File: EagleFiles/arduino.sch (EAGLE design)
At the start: 41 parts, among them IC1 4067D, IC2 4067D, IC3 4067D, J1 AVR_SPI, U1 ATMEGA168

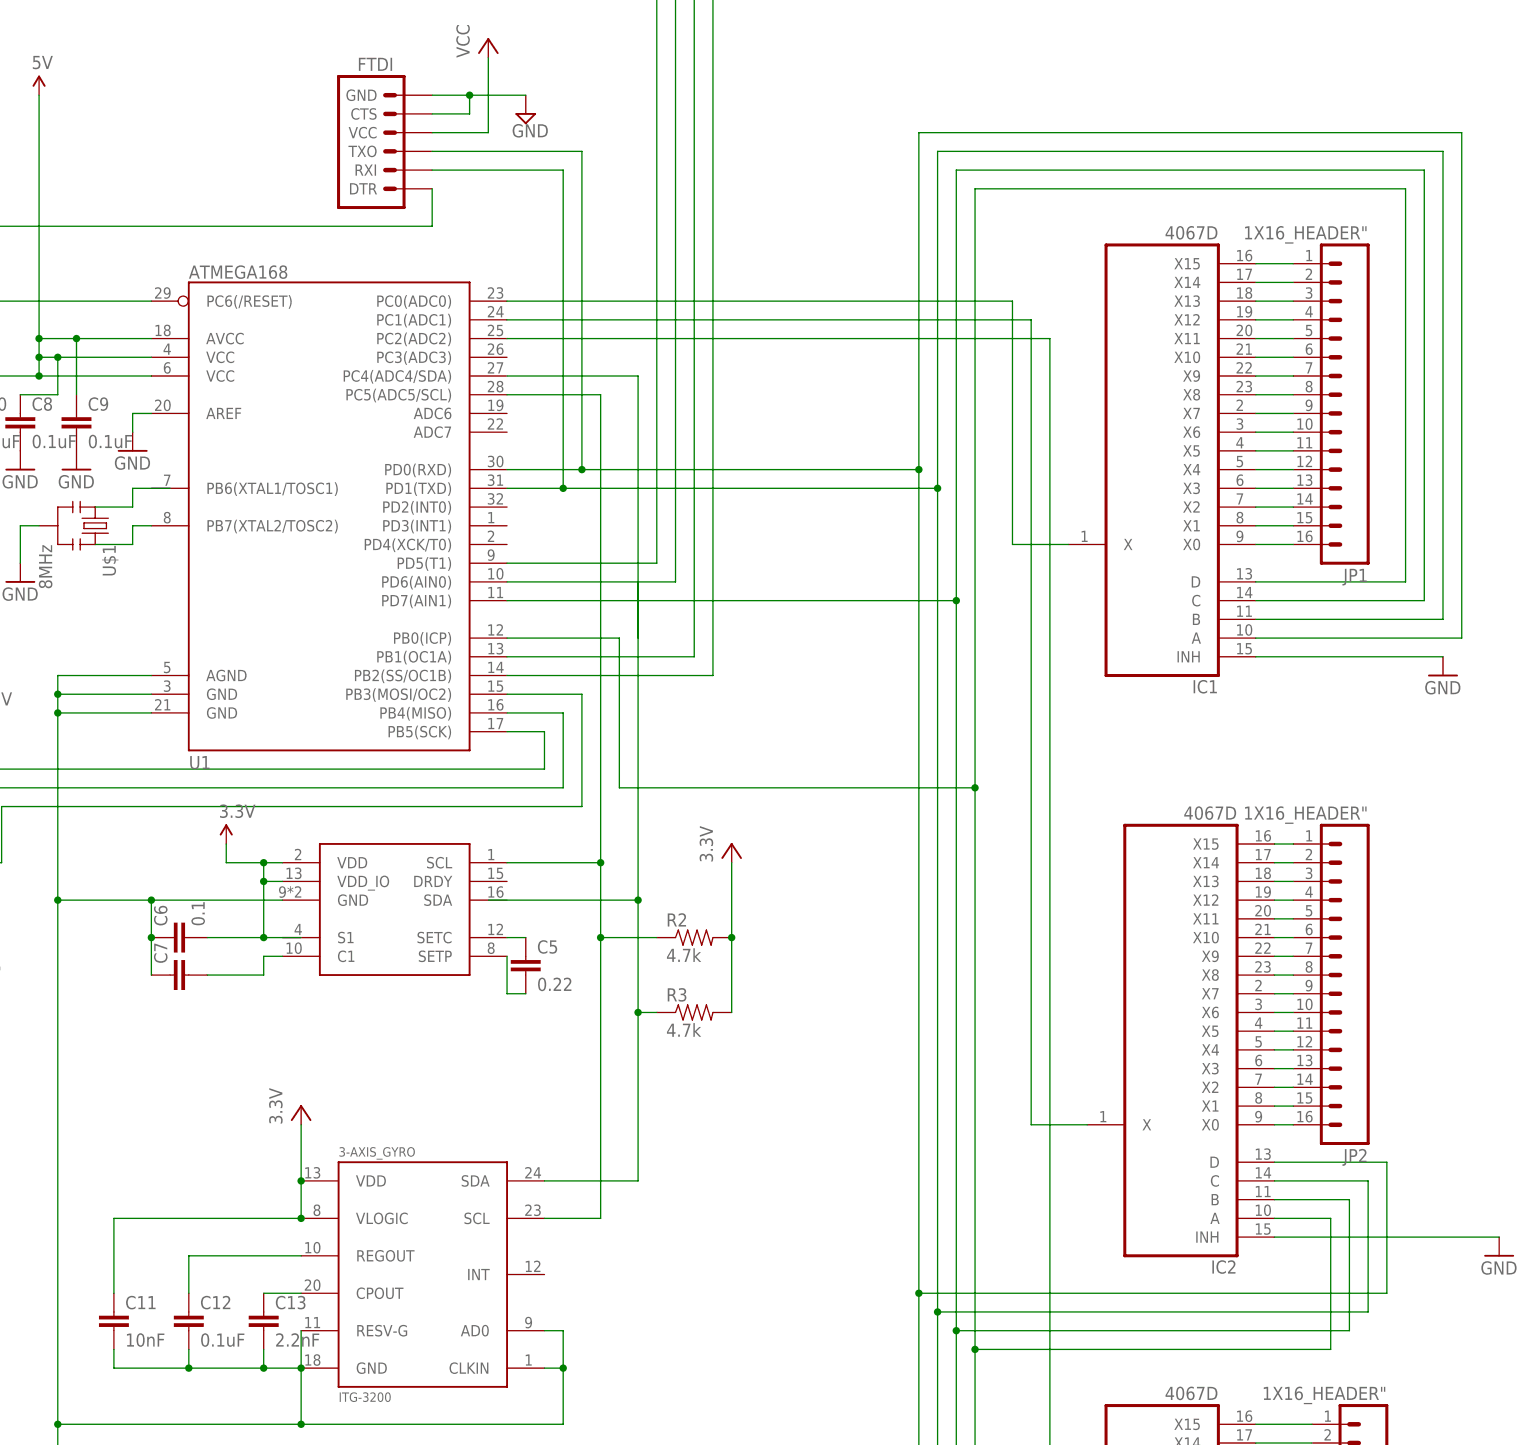
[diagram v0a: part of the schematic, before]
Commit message: made some changes?
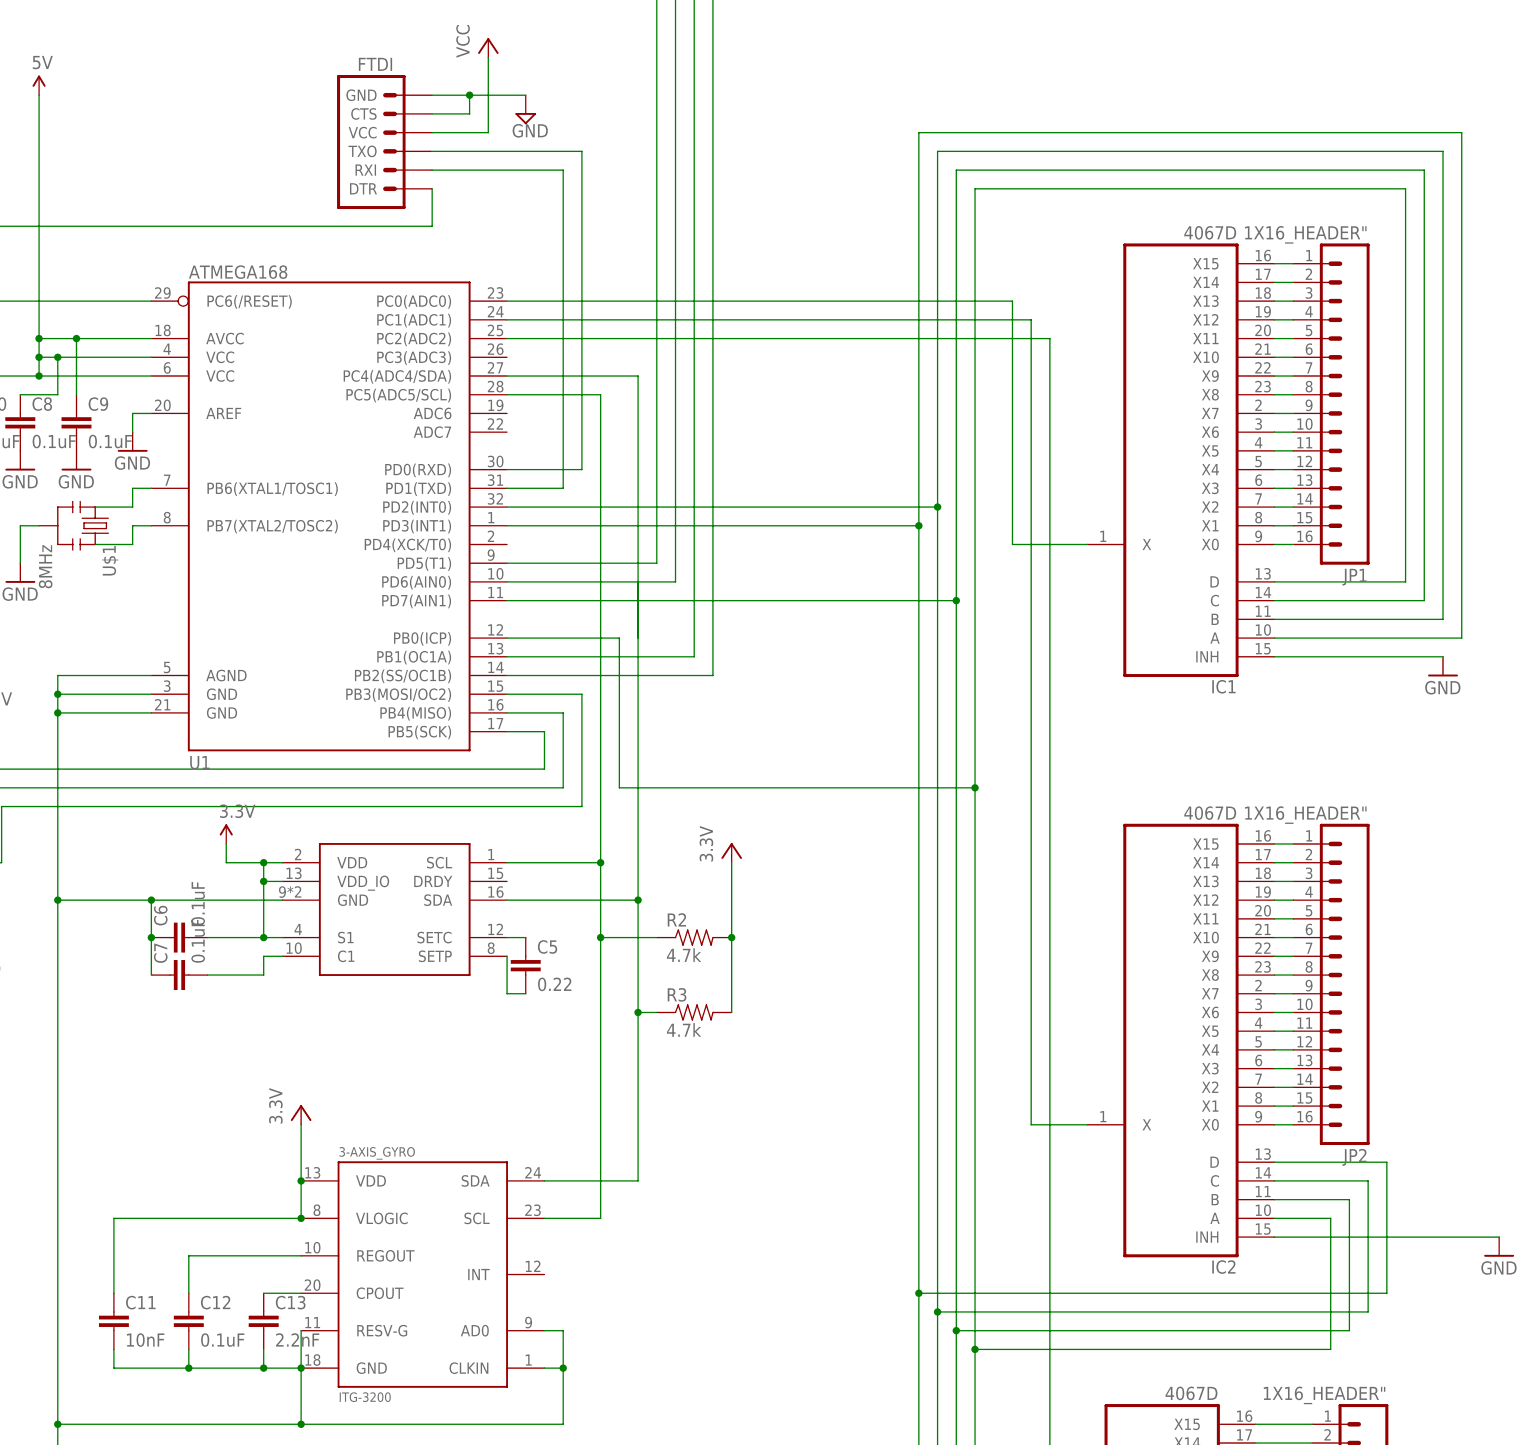
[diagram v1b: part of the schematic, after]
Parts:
- C6: value 0.1 -> 0.1uF
- C7: value (none) -> 0.1uF
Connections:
- new net N$80: FTDI.TXO, U1.PD0(RXD)
- new net N$81: FTDI.RXI, U1.PD1(TXD)
- net N$3: now also U1.PD2(INT0); no longer FTDI.RXI, U1.PD1(TXD)
- net N$4: now also U1.PD3(INT1); no longer FTDI.TXO, U1.PD0(RXD)
- net N$43: now also 3-AXIS_MAG.SDA
- net N$69: now also U1.PB6(XTAL1/TOSC1)
- net VCC: now also 3-AXIS_MAG.S1
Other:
- moved on the sheet: IC1
